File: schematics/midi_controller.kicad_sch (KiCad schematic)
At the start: 14 parts, among them U1 4051, U2 Teensy4.0

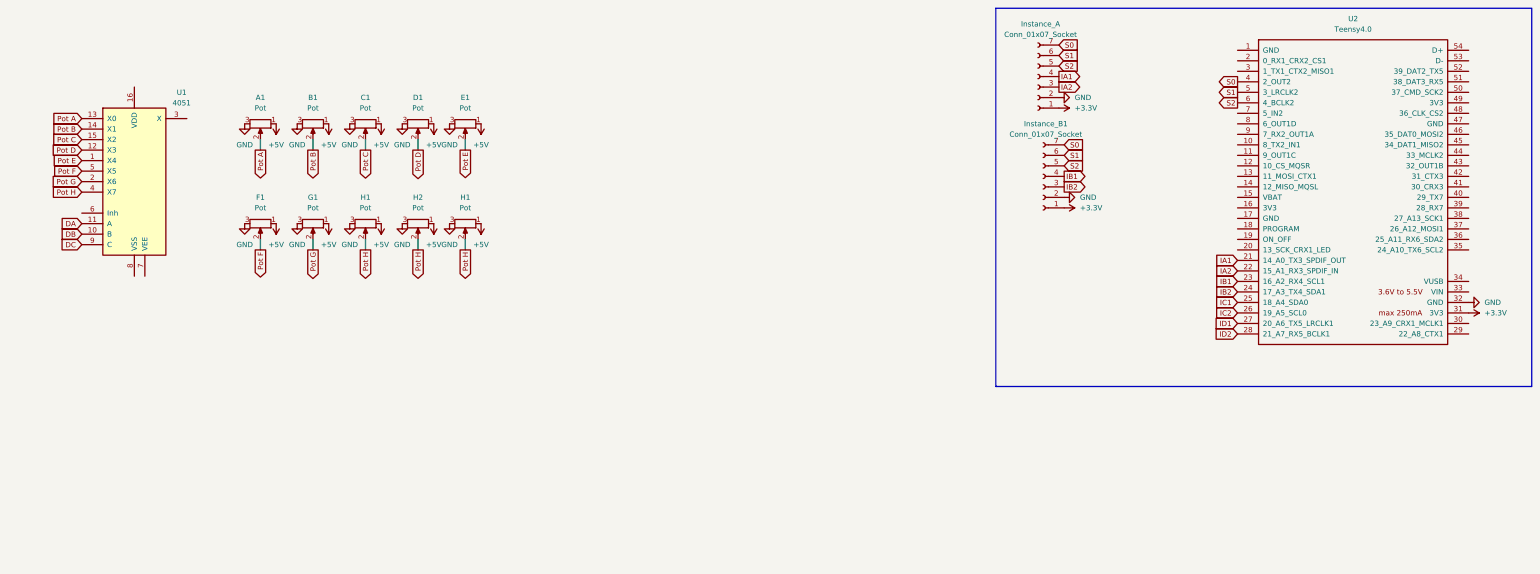
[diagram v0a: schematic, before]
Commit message: fixing stuff
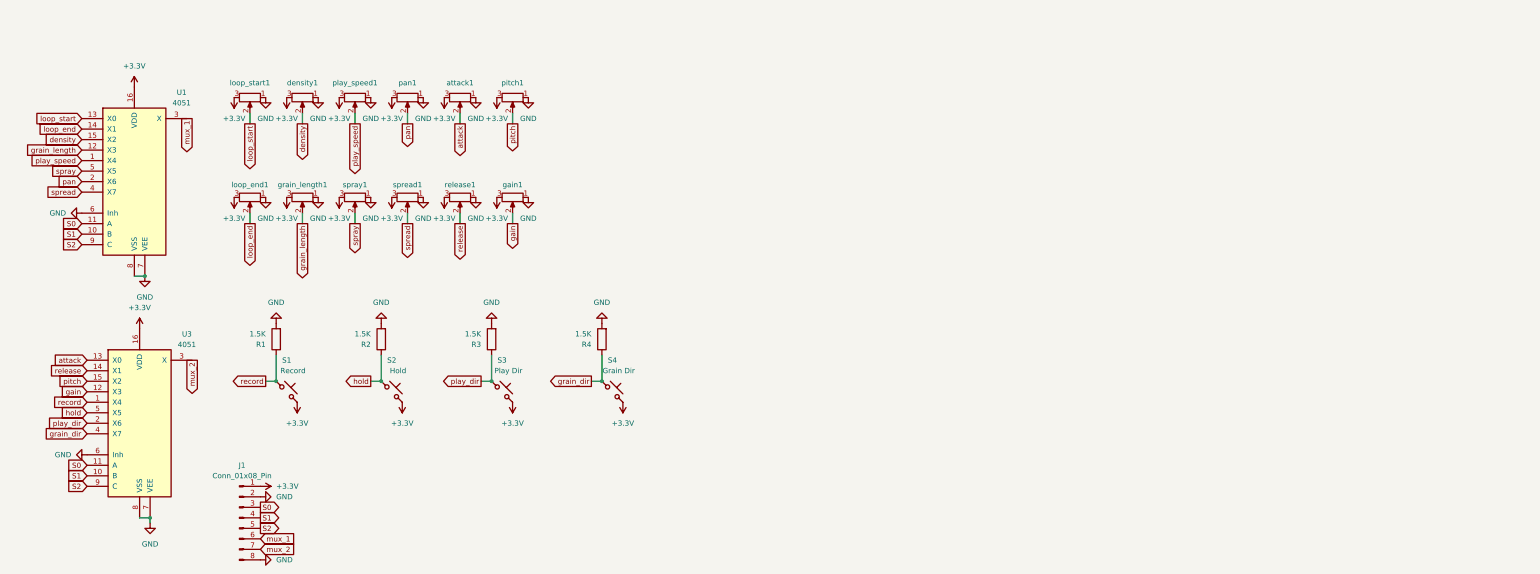
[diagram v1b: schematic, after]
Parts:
- removed G1, H1 (x2), H2: Pot, Potentiometer_THT:Potentiometer_TT_P0915N, symbol Device:R_Potentiometer
- removed Instance_A, Instance_B1: Conn_01x07_Socket, symbol Connector:Conn_01x07_Socket
- removed U2: Teensy4.0, symbol teensy:Teensy4.0
- added J1: Conn_01x08_Pin, Connector_IDC:IDC-Header_2x04_P2.54mm_Vertical, symbol Connector:Conn_01x08_Pin
- added R1, R2, R3, R4: 1.5K, Resistor_THT:R_Axial_DIN0204_L3.6mm_D1.6mm_P5.08mm_Horizontal, symbol Device:R
- added S1: Record, Button_Switch_Keyboard:SW_Cherry_MX_1.00u_PCB, symbol ScottoKeebs:Placeholder_Keyswitch
- added S2: Hold, Button_Switch_Keyboard:SW_Cherry_MX_1.00u_PCB, symbol ScottoKeebs:Placeholder_Keyswitch
- added S3: Play Dir, Button_Switch_Keyboard:SW_Cherry_MX_1.00u_PCB, symbol ScottoKeebs:Placeholder_Keyswitch
- added S4: Grain Dir, Button_Switch_Keyboard:SW_Cherry_MX_1.00u_PCB, symbol ScottoKeebs:Placeholder_Keyswitch
- added U3: 4051, Package_DIP:DIP-16_W7.62mm_Socket, symbol 4xxx:4051
- added gain1, grain_length1, loop_end1, release1, spray1, spread1: ~, Potentiometer_THT:Potentiometer_TT_P0915N, symbol Device:R_Potentiometer
- attack1: renamed from E1; value Pot -> ~
- density1: renamed from B1; value Pot -> ~
- loop_start1: renamed from A1; value Pot -> ~
- pan1: renamed from D1; value Pot -> ~
- pitch1: renamed from F1; value Pot -> ~
- play_speed1: renamed from C1; value Pot -> ~
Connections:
- net +5V is gone; now on net GND: attack1.1, density1.1, loop_start1.1, pan1.1, pitch1.1, play_speed1.1
- net DA is gone; now on net S0: U1.11 (A)
- net DB is gone; now on net S1: U1.10 (B)
- net DC is gone; now on net S2: U1.9 (C)
- net +3.3V: now also U1.16 (VDD), attack1.3, density1.3, loop_start1.3, pan1.3, pitch1.3, play_speed1.3, J1.1 (Pin_1), S1.2, S2.2, S3.2, S4.2, U3.16 (VDD), gain1.3, grain_length1.3, loop_end1.3, release1.3, spray1.3, spread1.3
- net GND: now also U1.6 (Inh), U1.7 (VEE), U1.8 (VSS), J1.2 (Pin_2), J1.8 (Pin_8), R1.2, R2.2, R3.2, R4.2, U3.6 (Inh), U3.7 (VEE), U3.8 (VSS), gain1.1, grain_length1.1, loop_end1.1, release1.1, spray1.1, spread1.1; no longer attack1.3, density1.3, loop_start1.3, pan1.3, pitch1.3, play_speed1.3
- net S0: now also J1.3 (Pin_3), U3.11 (A)
- net S1: now also J1.4 (Pin_4), U3.10 (B)
- net S2: now also J1.5 (Pin_5), U3.9 (C)
- net mux_1: now reaches U1.3 (X)
- net mux_1: now also J1.6 (Pin_6)
- net Pot A renamed loop_start
- net Pot B renamed density
- net density: now also U1.15 (X2); no longer U1.14 (X1)
- net Pot C renamed play_speed
- net play_speed: now also U1.1 (X4); no longer U1.15 (X2)
- net Pot D renamed grain_length
- net grain_length: now also grain_length1.2; no longer pan1.2
- net Pot E renamed attack
- net attack: now also U3.13 (X0); no longer U1.1 (X4)
- net Pot F renamed pitch
- net pitch: now also U3.15 (X2); no longer U1.5 (X5)
- net Pot G renamed pan
- net pan: now also pan1.2
- net Pot H renamed spread
- net spread: now also spread1.2
- new net gain: U3.12 (X3), gain1.2
- new net grain_dir: R4.1, S4.1, U3.4 (X7)
- new net hold: R2.1, S2.1, U3.5 (X5)
- new net loop_end: U1.14 (X1), loop_end1.2
- new net mux_2: J1.7 (Pin_7), U3.3 (X)
- new net play_dir: R3.1, S3.1, U3.2 (X6)
- new net record: R1.1, S1.1, U3.1 (X4)
- new net release: U3.14 (X1), release1.2
- new net spray: U1.5 (X5), spray1.2
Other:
- moved on the sheet: attack1, density1, loop_start1, pan1, pitch1, play_speed1
